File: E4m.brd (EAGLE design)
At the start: 50 x 100 mm, 78 parts, among them Q1 IRL540, Q2 IRL540, Q3 tip120

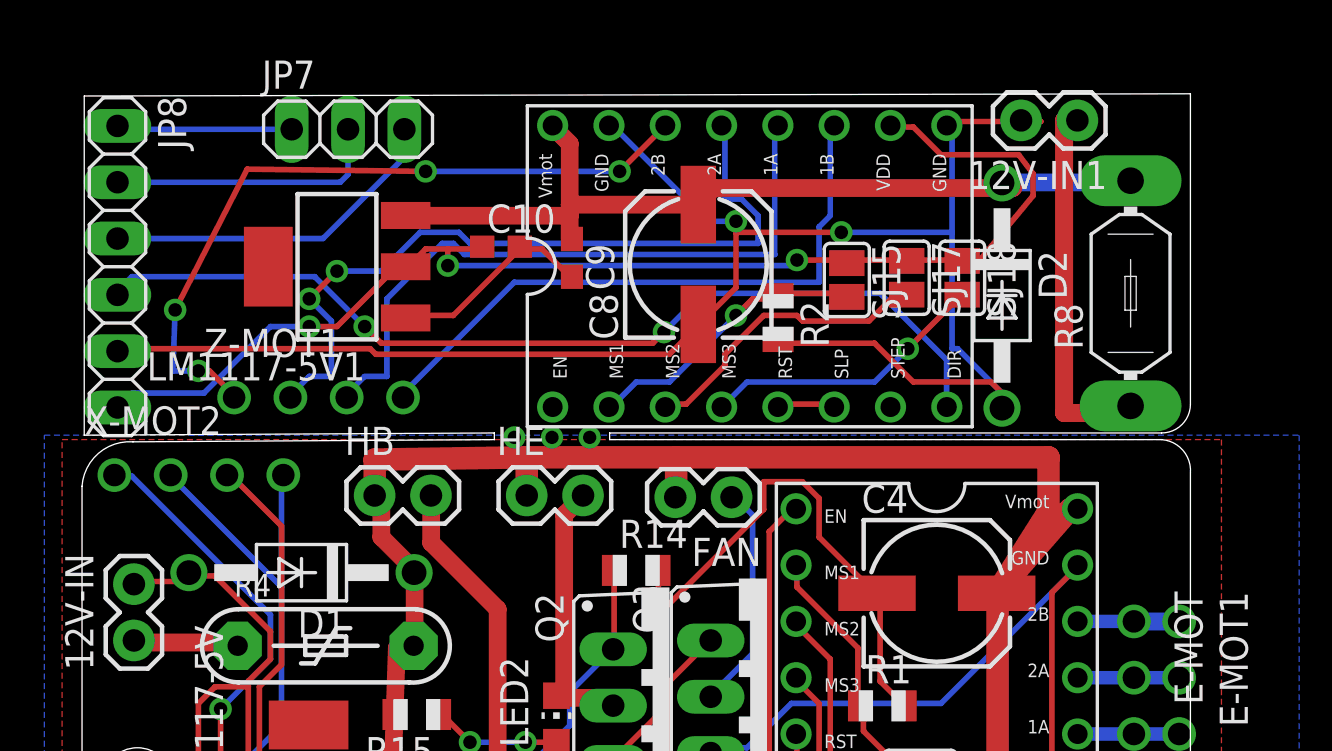
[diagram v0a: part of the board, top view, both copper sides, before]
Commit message: final?
mini4motion  esp4motion
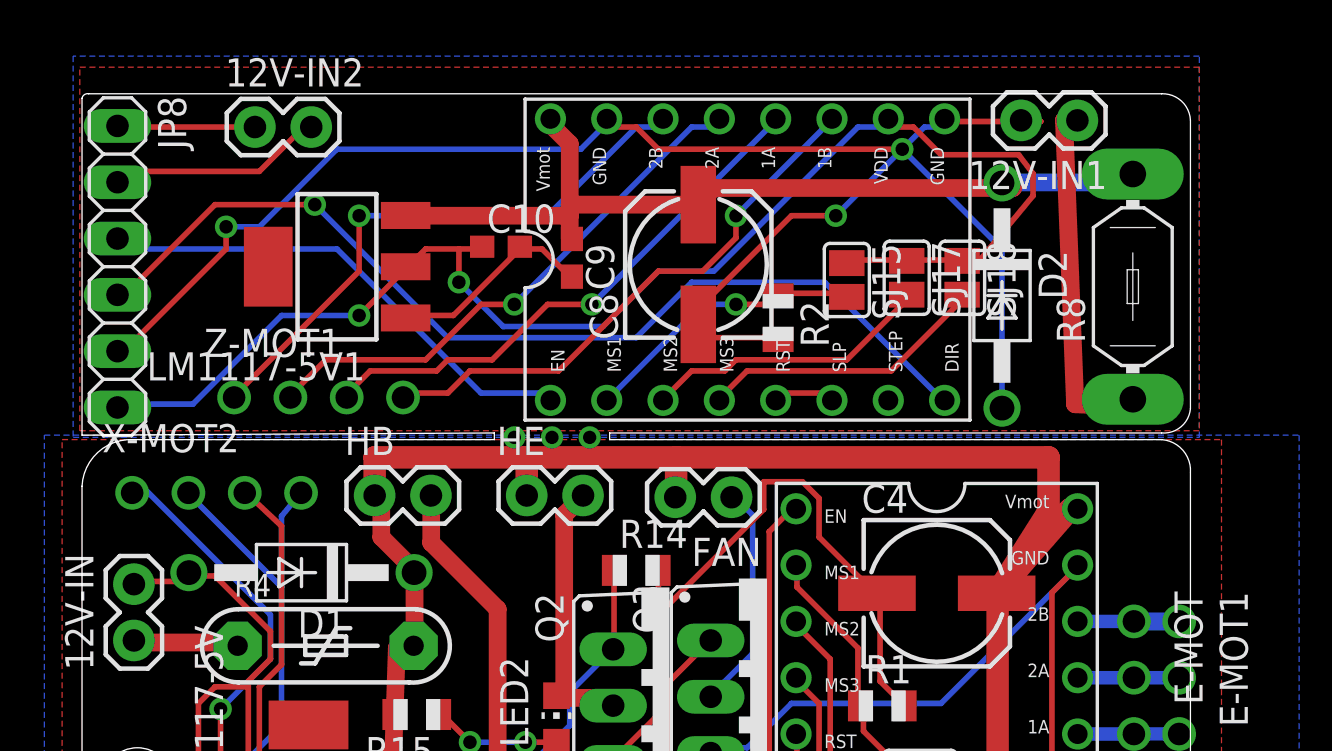
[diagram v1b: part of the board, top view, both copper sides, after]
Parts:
- removed JP7: (no value), pinhead:1X03
- added 12V-IN2: (no value), SparkFun:1X02
- moved X-MOT2 1.13 mm to (4.80, 82.0)
- moved R8 0.32 mm to (47.4, 91.3)
- moved U$6 0.32 mm to (22.4, 97.6)
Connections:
- removed net N$51: JP7.3, JP8.3
- net ENABLE1: now also JP8.3
- net N$52: now also 12V-IN2.2; no longer JP7.2
- net N$53: now also 12V-IN2.1; no longer JP7.1
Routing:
- net ENABLE1: track 0.00 -> 22.7 mm
- net N$51: track 15.7 -> 0.00 mm
- net N$42: track 34.4 -> 24.6 mm, vias 2 -> 1
- net 5V1: track 56.7 -> 63.7 mm, vias 3 -> 2
- net N$41: track 32.9 -> 26.1 mm, vias 4 -> 1
- net N$43: track 30.4 -> 24.6 mm, vias 0 -> 1
- net N$44: track 28.4 -> 25.3 mm, vias 0 -> 1
- net N$52: track 12.6 -> 9.80 mm
- net GND1: track 81.7 -> 78.9 mm, vias 2 -> 3
- net N$53: track 8.90 -> 6.49 mm
- net ANALOG: track 71.9 -> 70.5 mm
- net S-A0: track 39.7 -> 38.7 mm
- net Z-DIR1: track 43.6 -> 44.7 mm, vias 2 -> 1
- net S-A1: track 43.2 -> 42.2 mm
- net N$47: track 17.1 -> 16.2 mm
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- added copper zone on layer 1, net GND1
- added copper zone on layer 16, net GND1
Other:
- outline, holes or cut-outs redrawn
